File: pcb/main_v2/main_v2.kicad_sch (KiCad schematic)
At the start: 1 part, among them J102 Conn_02x06_Odd_Even

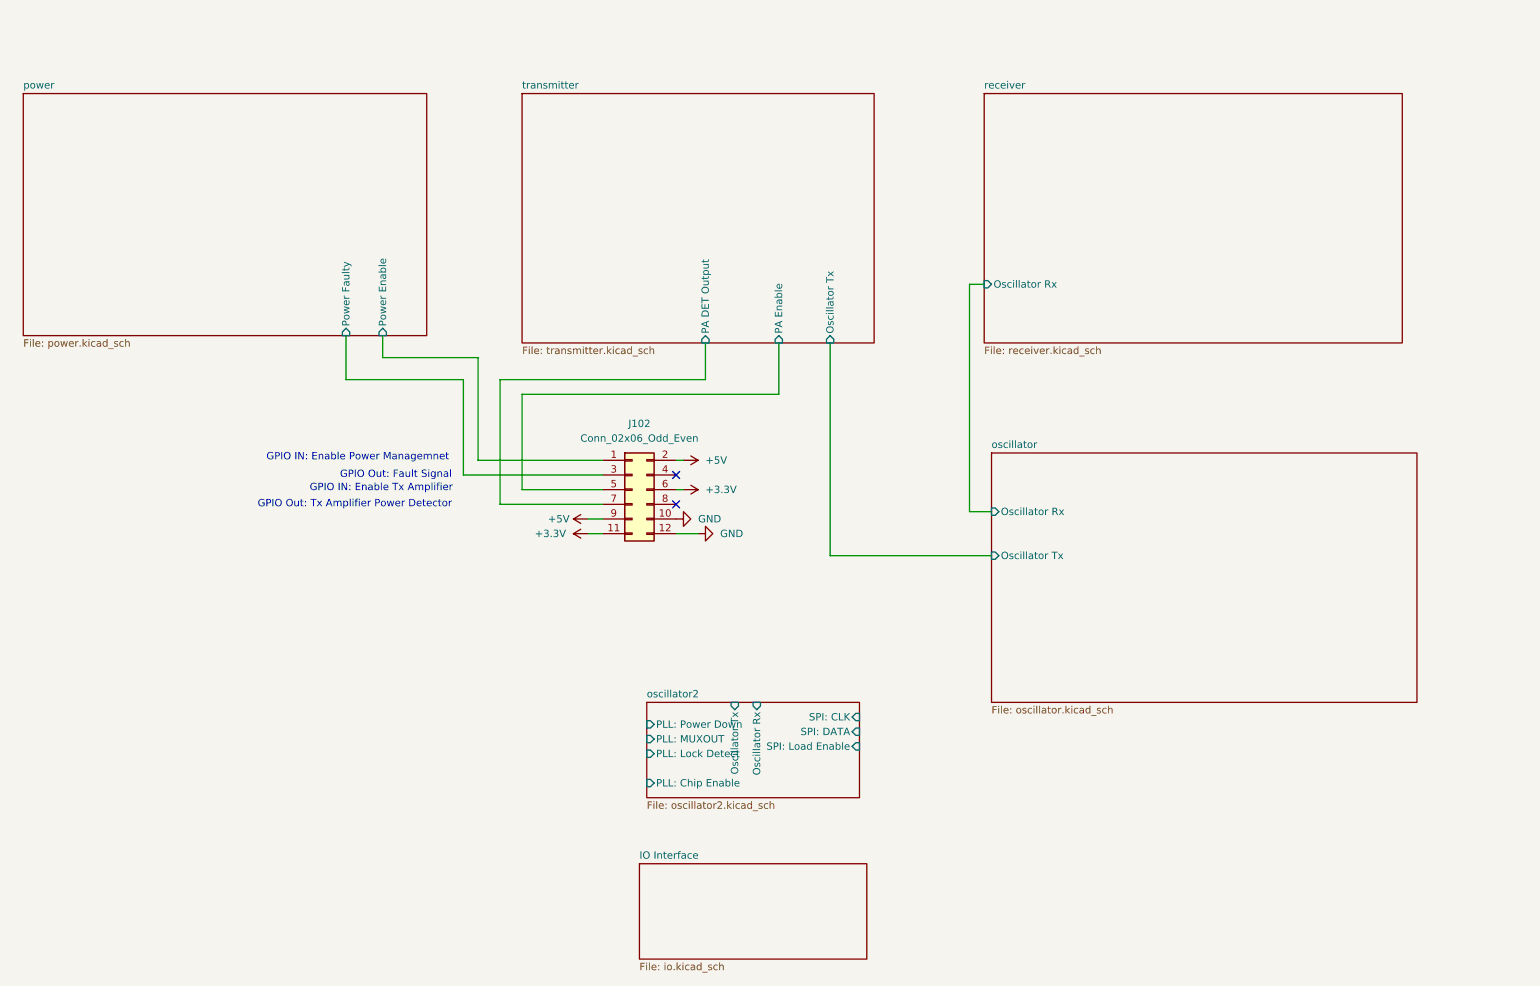
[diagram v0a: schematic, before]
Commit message: updarted schematic and simulation
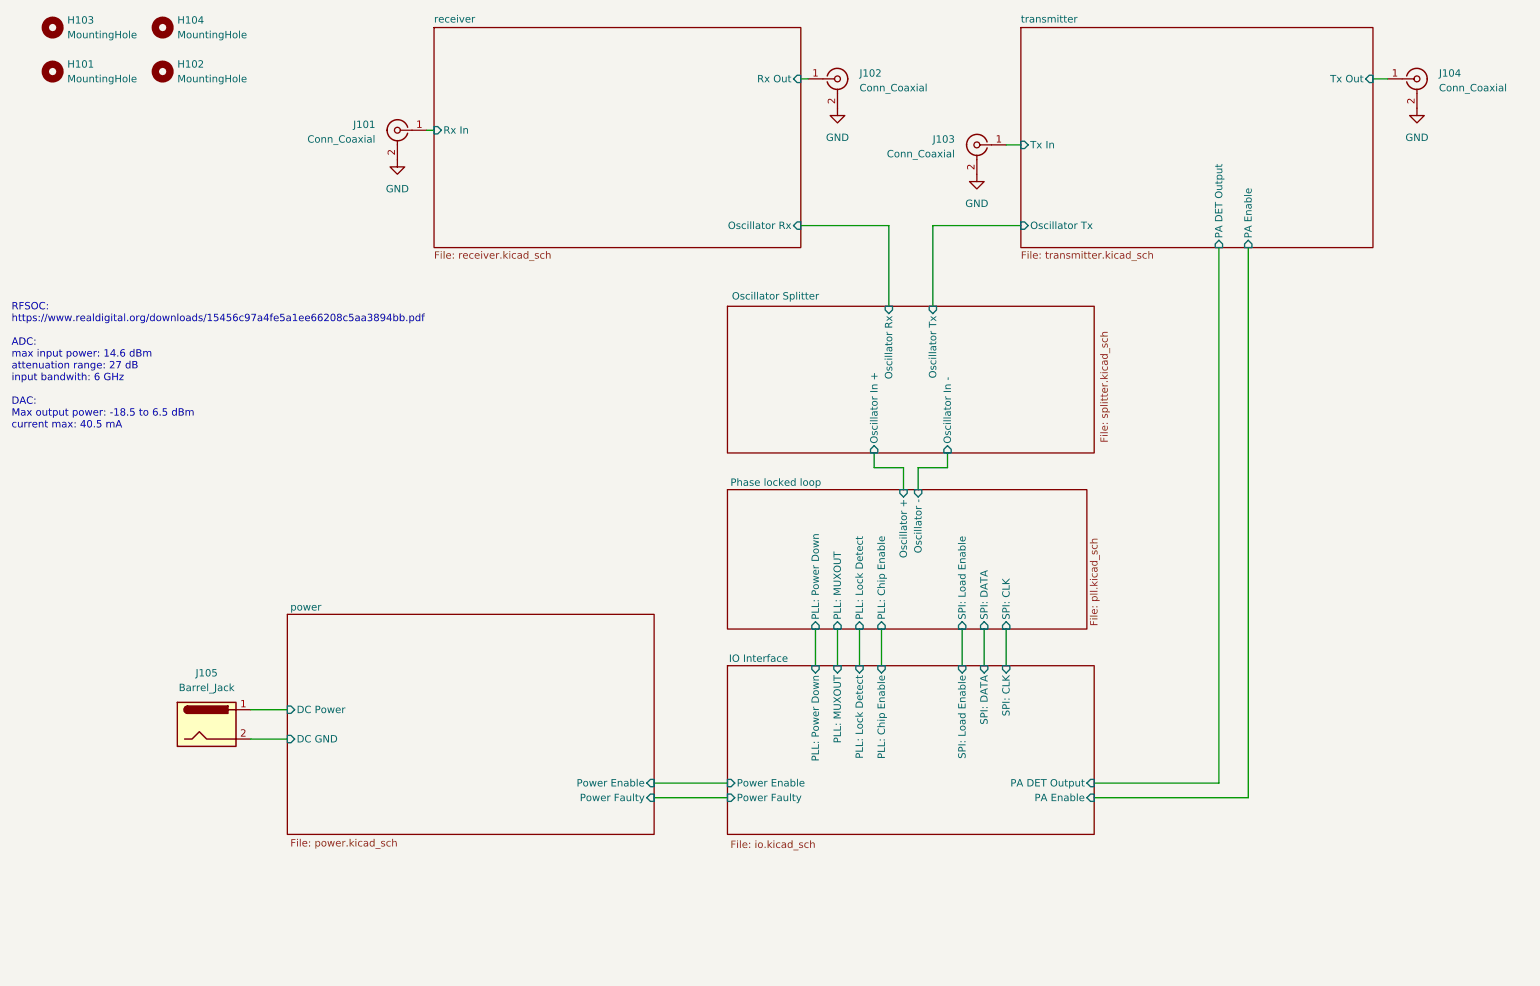
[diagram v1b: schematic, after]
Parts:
- removed J102: Conn_02x06_Odd_Even, symbol Connector_Generic:Conn_02x06_Odd_Even
- added H101, H102, H103, H104: MountingHole, MountingHole:MountingHole_2.2mm_M2, symbol Mechanical:MountingHole
- added J101, J102, J103, J104: Conn_Coaxial, Connector_Coaxial:SMA_Amphenol_132289_EdgeMount, symbol Connector:Conn_Coaxial
- added J105: Barrel_Jack, Connector_BarrelJack:BarrelJack_CUI_PJ-063AH_Horizontal_CircularHoles, symbol Connector:Barrel_Jack
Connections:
- net GND: now also J101.2 (Ext), J102.2 (Ext), J103.2 (Ext), J104.2 (Ext)
- new net power/DC GND: J105.2
- new net power/DC Power: J105.1
- new net receiver/Rx In: J101.1 (In)
- new net receiver/Rx Out: J102.1 (In)
- new net transmitter/Tx In: J103.1 (In)
- new net transmitter/Tx Out: J104.1 (In)
- no-connect marks 2 -> 0
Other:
- sheet oscillator2 renamed Phase locked loop
- removed sheet oscillator
- added sheet Oscillator Splitter (splitter.kicad_sch)
- sheet IO Interface ports: added PA DET Output, PA Enable, PLL: Chip Enable, PLL: Lock Detect, PLL: MUXOUT, PLL: Power Down, Power Enable, Power Faulty, SPI: CLK, SPI: DATA, SPI: Load Enable; removed none
- sheet Phase locked loop: file oscillator2.kicad_sch -> pll.kicad_sch
- sheet Phase locked loop ports: added Oscillator +, Oscillator -; removed Oscillator Rx, Oscillator Tx
- sheet power ports: added DC GND, DC Power; removed none
- sheet receiver ports: added Rx In, Rx Out; removed none
- sheet transmitter ports: added Tx In, Tx Out; removed none
- note added: "RFSOC: https://www.realdigital.org/downloads/15456c97a4fe5a1ee66208c5aa3894bb.pdf ADC: max input power: 14.6 dBm attenuation range: 27 dB input bandwith: 6 GHz DAC: Max output power: -18.5 to 6.5 dBm current max: 40.5 mA"
- note removed: "GPIO IN: Enable Power Managemnet"
- note removed: "GPIO IN: Enable Tx Amplifier"
- note removed: "GPIO Out: Fault Signal"
- note removed: "GPIO Out: Tx Amplifier Power Detector"
